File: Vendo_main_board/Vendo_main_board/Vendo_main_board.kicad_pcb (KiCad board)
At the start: 2 copper layers, 60 x 100 mm, 117 parts, among them J1 Screw_Terminal_01x04, J10 Screw_Terminal_01x03, J11 Screw_Terminal_01x02, J12 Screw_Terminal_01x03, J2 Barrel_Jack_MountingPin, J3 Conn_01x05_Pin, J4 Conn_01x05_Pin, J5 BOOT, J6 Screw_Terminal_01x04, J7 FTDI, J9 Conn_01x04_Pin, Q1 Q_NMOS_Depletion_GSD, Q2 Q_NMOS_Depletion_GSD, Q3 Q_NMOS_Depletion_GSD, Q4 Q_NMOS_Depletion_GSD, SW1 SW_Push, SW2 SW_Push, SW3 SW_Push, SW4 SW_Push, SW5 SW_Slide_DPDT, U1 AMS1117-3.3, U2 AP64350SP-13, U3 STM32F103C8T6, U4 PC817, Y1 32.768kHz, Y2 8MHz

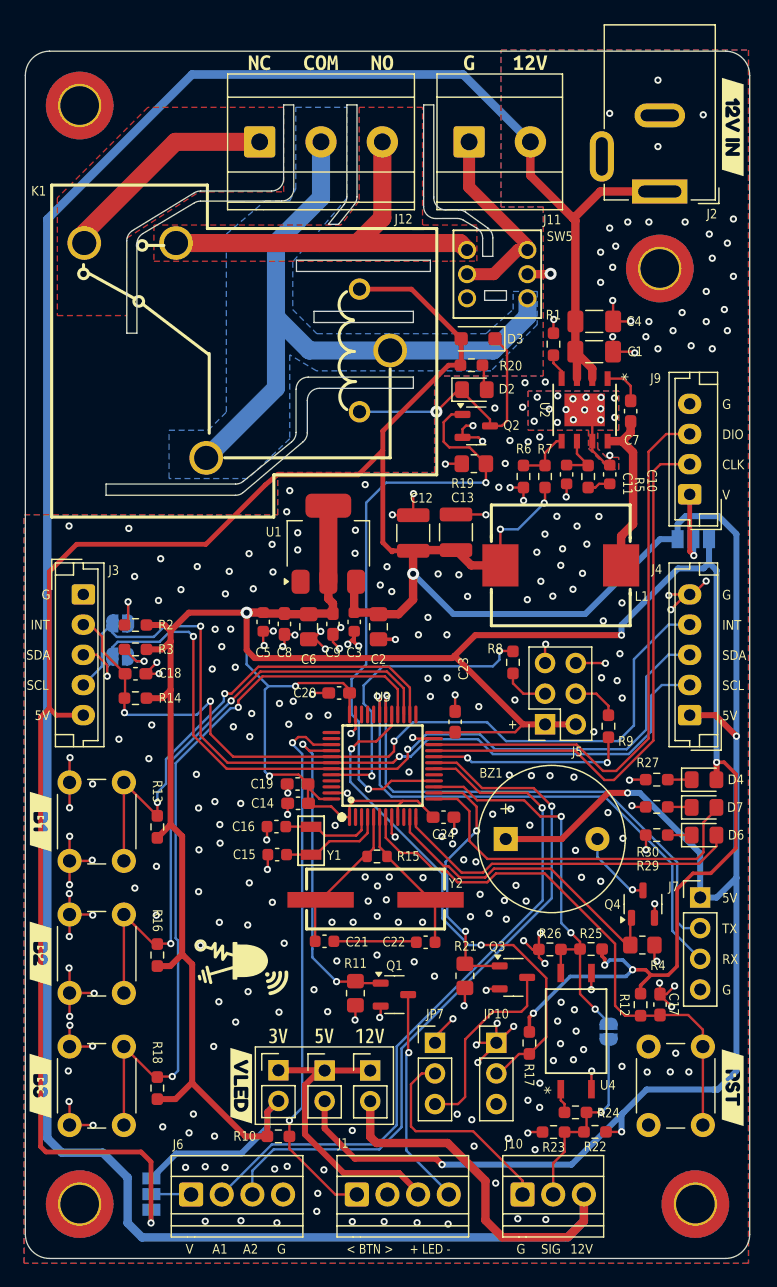
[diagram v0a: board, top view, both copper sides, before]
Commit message: -repush
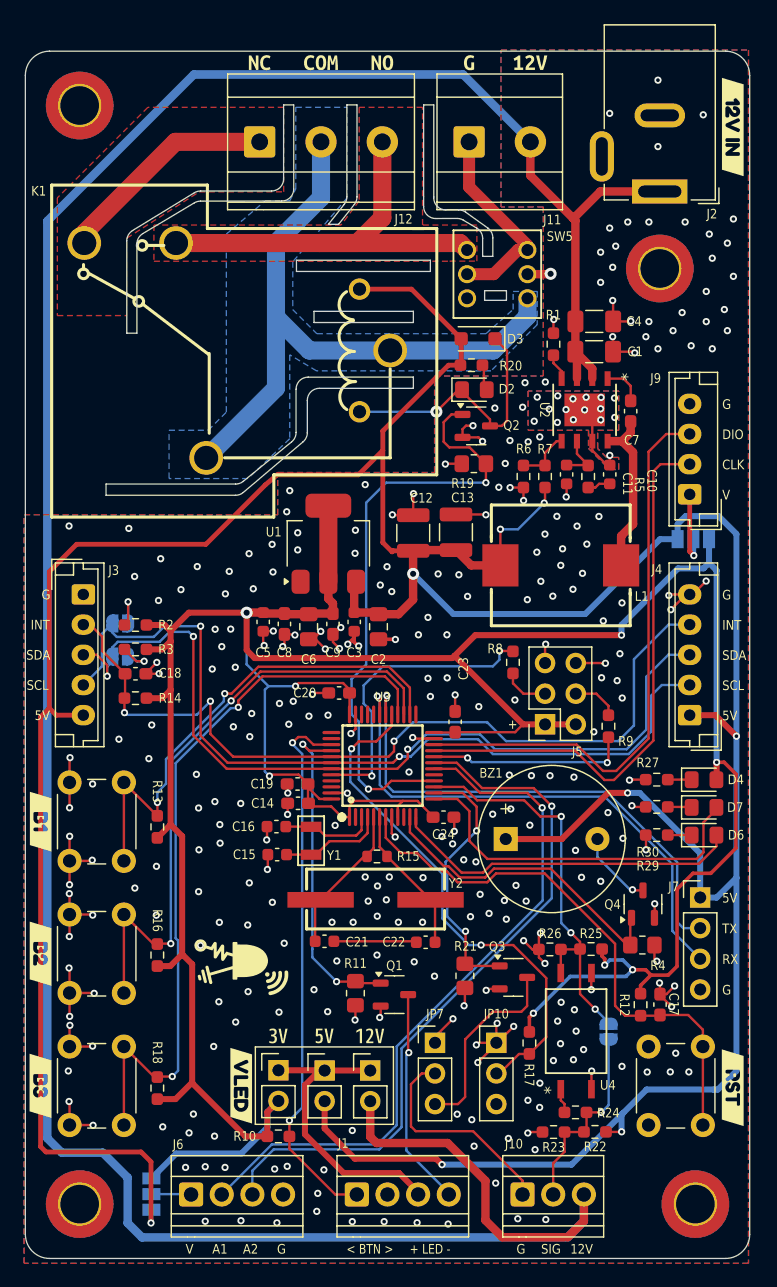
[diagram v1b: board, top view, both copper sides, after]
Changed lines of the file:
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@@
 	)
 	(segment
-		(start 234.355 29.53)
-		(end 211.91 29.53)
+		(start 212.06 29.53)
+		(end 199.92 41.67)
 		(width 0.7)
 		(layer "B.Cu")
@@
 	)
 	(segment
-		(start 211.91 29.53)
-		(end 199.92 41.52)
+		(start 199.92 41.67)
+		(end 199.92 117.64)
+		(width 0.7)
+		(layer "B.Cu")
+		(net 1)
+	)
+	(segment
+		(start 206.57 120.9)
+		(end 206.57 124.66)
+		(width 0.7)
+		(layer "B.Cu")
+		(net 1)
+	)
+	(segment
+		(start 234.355 29.53)
+		(end 212.06 29.53)
+		(width 0.7)
+		(layer "B.Cu")
+		(net 1)
+	)
+	(segment
+		(start 244.3625 124.5175)
+		(end 244.3625 122.3025)
+		(width 0.7)
+		(layer "B.Cu")
+		(net 1)
+	)
+	(segment
+		(start 243.02 125.86)
+		(end 244.3625 124.5175)
+		(width 0.7)
+		(layer "B.Cu")
+		(net 1)
+	)
+	(segment
+		(start 239.935 35.11)
+		(end 234.355 29.53)
 		(width 0.7)
 		(layer "B.Cu")
@@
 	)
 	(segment
-		(start 239.935 35.11)
-		(end 234.355 29.53)
+		(start 204.51 118.84)
+		(end 206.57 120.9)
 		(width 0.7)
 		(layer "B.Cu")
@@
 	)
 	(segment
-		(start 204.51 118.84)
-		(end 206.57 120.9)
-		(width 0.7)
-		(layer "B.Cu")
-		(net 1)
-	)
-	(segment
-		(start 206.57 120.9)
-		(end 206.57 124.66)
-		(width 0.7)
-		(layer "B.Cu")
-		(net 1)
-	)
-	(segment
-		(start 199.92 41.52)
-		(end 199.92 117.64)
-		(width 0.7)
-		(layer "B.Cu")
-		(net 1)
-	)
-	(segment
-		(start 244.3625 124.5175)
-		(end 244.3625 122.3025)
+		(start 206.57 124.66)
+		(end 207.77 125.86)
 		(width 0.7)
 		(layer "B.Cu")
@@
 		(width 0.7)
 		(layer "B.Cu")
-		(net 1)
-	)
-	(segment
-		(start 206.57 124.66)
-		(end 207.77 125.86)
-		(width 0.7)
-		(layer "B.Cu")
-		(net 1)
-	)
-	(segment
-		(start 243.02 125.86)
-		(end 244.3625 124.5175)
-		(width 0.7)
-		(layer "B.Cu")
